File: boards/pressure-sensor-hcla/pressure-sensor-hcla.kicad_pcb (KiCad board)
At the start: 2 copper layers, 27.5 x 19 mm, 5 parts, among them J1 CONN_01X04, M3 MountingHole_3.2mm_M3, U1 HCLA-XXXX-DIP-X

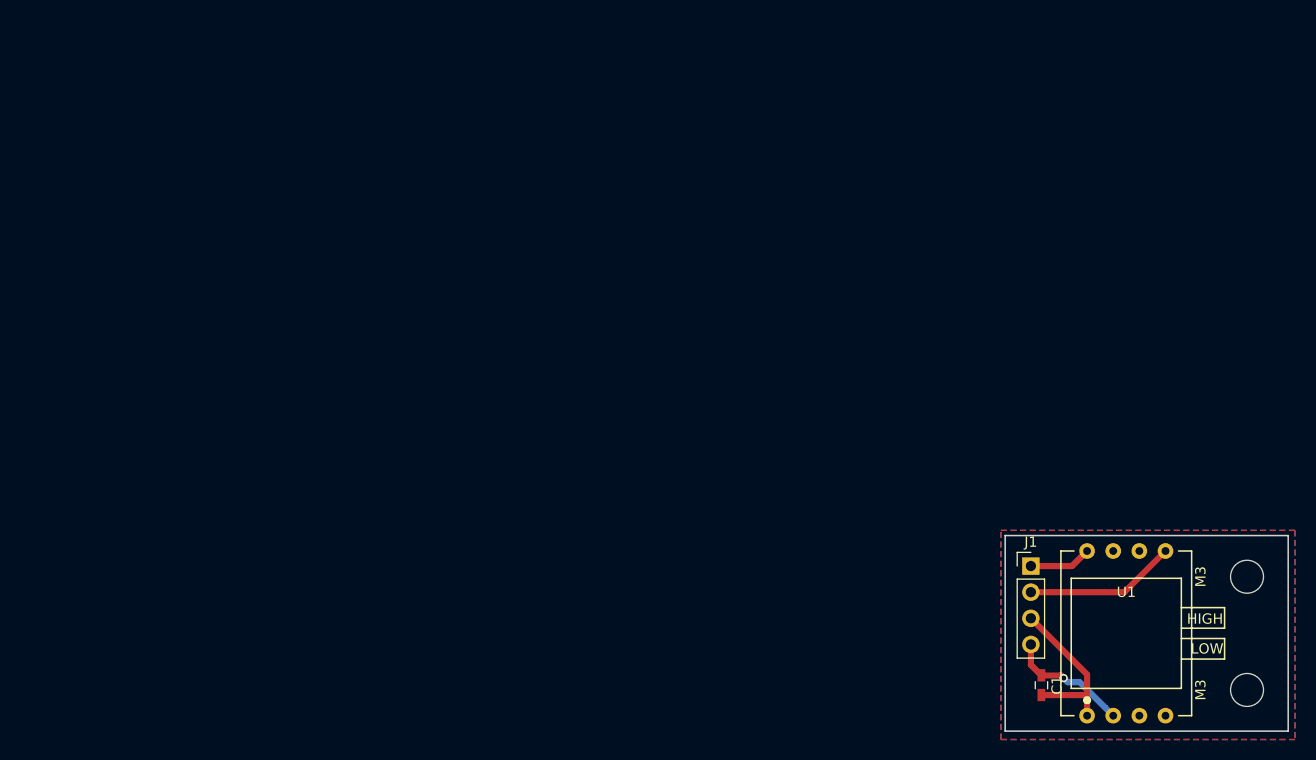
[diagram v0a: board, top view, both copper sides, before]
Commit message: [docs] export all board layouts
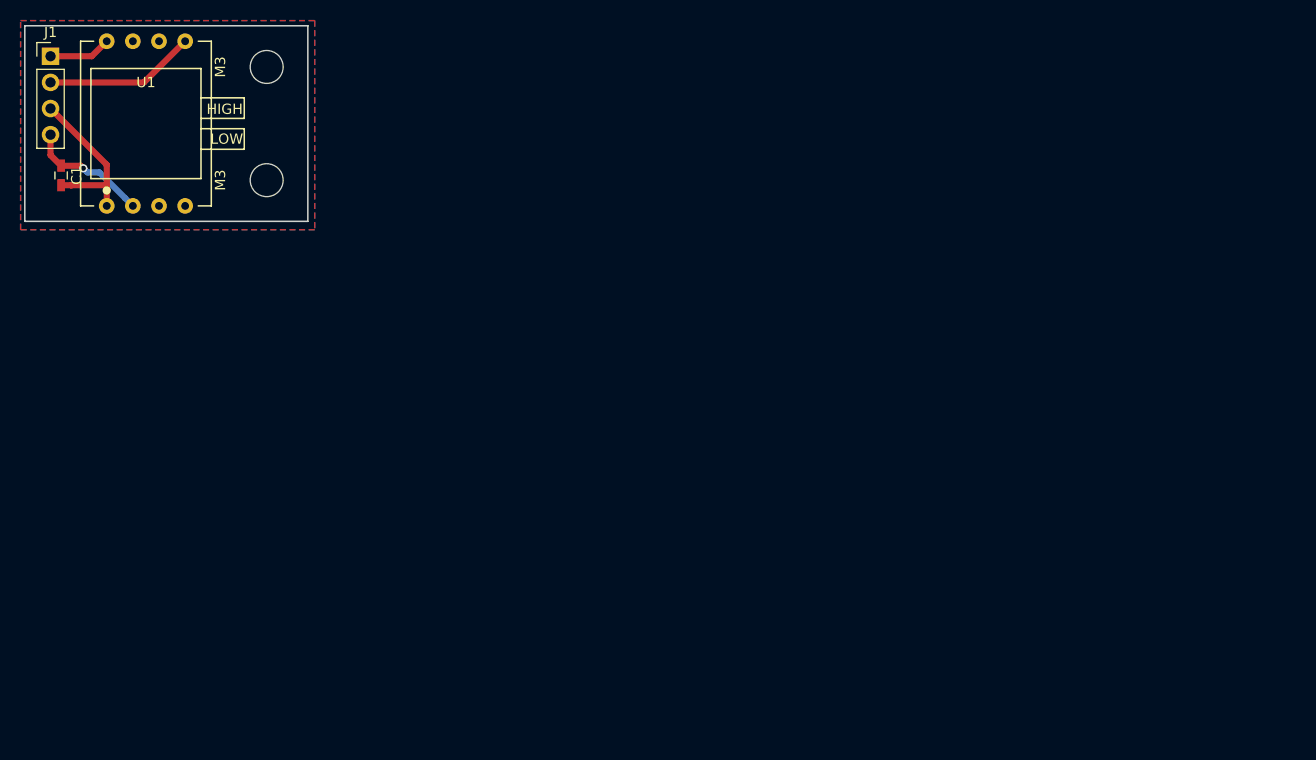
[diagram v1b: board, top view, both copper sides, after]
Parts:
- moved J1 107.4 mm to (56.2, 40.9)
- moved M3 107.4 mm to (77.2, 42.0)
- moved M3 107.4 mm to (77.2, 53.0)
- moved C1 107.4 mm to (57.3, 52.5)
- moved U1 107.4 mm to (59.2, 55.5)
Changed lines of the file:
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@@
   (general
     (links 6)
-    (no_connects 1)
+    (no_connects 0)
     (area 147.025 85.525 182.057143 109.075)
     (thickness 1.6)
@@
     (nets 5)
   )
-  (page A4)
+  (page User 140.005 119.99)
+  (title_block
+    (title "Pressure sensor board HCLA")
+    (date 2017-05-21)
+    (rev 1)
+    (company VIPER)
+  )
   (layers
     (0 F.Cu signal)
@@
   )
   (module Capacitors_SMD:C_0603_HandSoldering (layer F.Cu)
-    (at 152.527 102.042 90)
+    (at 57.277 52.512 90)
     (descr "Capacitor SMD 0603, hand soldering")
     (tags "capacitor 0603")
@@
   )
   (module Pin_Headers:Pin_Header_Straight_1x04_Pitch2.54mm (layer F.Cu)
-    (at 151.5 90.46)
+    (at 56.25 40.93)
     (descr "Through hole straight pin header, 1x04, 2.54mm pitch, single row")
     (tags "Through hole pin header THT 1x04 2.54mm single row")
@@
   )
   (module pressure-sensor-hcla:HCLA-DIP (layer F.Cu)
-    (at 154.42 105)
+    (at 59.17 55.47)
     (fp_text reference U1 (at 6.35 -12) (layer F.SilkS)
       (effects (font (size 1 1) (thickness 0.15)))
@@
   )
   (module Mounting_Holes:MountingHole_3.2mm_M3 (layer F.Cu)
-    (at 172.5 91.5)
+    (at 77.25 41.97)
     (descr "Mounting Hole 3.2mm, no annular, M3")
     (tags "mounting hole 3.2mm no annular m3")
@@
   )
   (module Mounting_Holes:MountingHole_3.2mm_M3 (layer F.Cu)
-    (at 172.5 102.5)
+    (at 77.25 52.97)
     (descr "Mounting Hole 3.2mm, no annular, M3")
     (tags "mounting hole 3.2mm no annular m3")
@@
     (pad 1 np_thru_hole circle (at 0 0) (size 3.2 3.2) (drill 3.2) (layers *.Cu *.Mask))
   )
-  (gr_text GND (at 155.5 98.5) (layer B.SilkS)
-    (effects (font (size 1.5 1.5) (thickness 0.3)) (justify mirror))
-  )
-  (gr_text "rexus-viper\npressure-\nsensor-HCLA\n©rchojetzki" (at 163.5 97 90) (layer B.SilkS)
-    (effects (font (size 1.5 1.5) (thickness 0.3)) (justify mirror))
-  )
-  (gr_text VCC (at 155.5 95.5) (layer B.SilkS)
-    (effects (font (size 1.5 1.5) (thickness 0.3)) (justify mirror))
-  )
-  (gr_text SCL (at 155.5 93) (layer B.SilkS)
-    (effects (font (size 1.5 1.5) (thickness 0.3)) (justify mirror))
-  )
-  (gr_text SDA (at 155.5 90.5) (layer B.SilkS)
-    (effects (font (size 1.5 1.5) (thickness 0.3)) (justify mirror))
-  )
-  (gr_line (start 176.5 106.5) (end 176.5 87.5) (layer Edge.Cuts) (width 0.15))
-  (gr_line (start 149 106.5) (end 176.5 106.5) (layer Edge.Cuts) (width 0.15))
-  (gr_line (start 149 87.5) (end 149 106.5) (layer Edge.Cuts) (width 0.15))
-  (gr_line (start 176.5 87.5) (end 149 87.5) (layer Edge.Cuts) (width 0.15))
-  (segment (start 156.96 101) (end 156.96 102.997) (width 0.6) (layer F.Cu) (net 1))
-  (segment (start 156.96 102.997) (end 156.96 105) (width 0.6) (layer F.Cu) (net 1))
-  (segment (start 152.527 102.992) (end 153.502 102.992) (width 0.6) (layer F.Cu) (net 1))
-  (segment (start 153.502 102.992) (end 153.507 102.997) (width 0.6) (layer F.Cu) (net 1))
-  (segment (start 153.507 102.997) (end 156.96 102.997) (width 0.6) (layer F.Cu) (net 1))
-  (segment (start 151.5 95.54) (end 156.96 101) (width 0.6) (layer F.Cu) (net 1))
-  (segment (start 154.686 101.346) (end 155.085999 101.745999) (width 0.6) (layer B.Cu) (net 2))
-  (segment (start 155.085999 101.745999) (end 156.245999 101.745999) (width 0.6) (layer B.Cu) (net 2))
-  (segment (start 156.245999 101.745999) (end 158.738001 104.238001) (width 0.6) (layer B.Cu) (net 2))
-  (segment (start 158.738001 104.238001) (end 159.5 105) (width 0.6) (layer B.Cu) (net 2))
-  (segment (start 152.527 101.092) (end 154.432 101.092) (width 0.6) (layer F.Cu) (net 2))
-  (segment (start 154.432 101.092) (end 154.686 101.346) (width 0.6) (layer F.Cu) (net 2))
-  (via (at 154.686 101.346) (size 0.8) (drill 0.5) (layers F.Cu B.Cu) (net 2))
-  (segment (start 151.5 98.08) (end 151.5 100.065) (width 0.6) (layer F.Cu) (net 2))
-  (segment (start 151.5 100.065) (end 152.527 101.092) (width 0.6) (layer F.Cu) (net 2))
-  (segment (start 151.92 98.5) (end 151.5 98.08) (width 0.6) (layer F.Cu) (net 2))
-  (segment (start 151.5 90.46) (end 155.5 90.46) (width 0.6) (layer F.Cu) (net 3))
-  (segment (start 155.5 90.46) (end 156.96 89) (width 0.6) (layer F.Cu) (net 3))
-  (segment (start 151.5 93) (end 160.58 93) (width 0.6) (layer F.Cu) (net 4))
-  (segment (start 160.58 93) (end 164.58 89) (width 0.6) (layer F.Cu) (net 4))
+  (gr_text GND (at 60.25 48.97) (layer B.SilkS)
+    (effects (font (size 1.5 1.5) (thickness 0.3)) (justify mirror))
+  )
+  (gr_text "rexus-viper\npressure-\nsensor-HCLA\n©rchojetzki" (at 68.25 47.47 90) (layer B.SilkS)
+    (effects (font (size 1.5 1.5) (thickness 0.3)) (justify mirror))
+  )
+  (gr_text VCC (at 60.25 45.97) (layer B.SilkS)
+    (effects (font (size 1.5 1.5) (thickness 0.3)) (justify mirror))
+  )
+  (gr_text SCL (at 60.25 43.47) (layer B.SilkS)
+    (effects (font (size 1.5 1.5) (thickness 0.3)) (justify mirror))
+  )
+  (gr_text SDA (at 60.25 40.97) (layer B.SilkS)
+    (effects (font (size 1.5 1.5) (thickness 0.3)) (justify mirror))
+  )
+  (gr_line (start 81.25 56.97) (end 81.25 37.97) (layer Edge.Cuts) (width 0.15))
+  (gr_line (start 53.75 56.97) (end 81.25 56.97) (layer Edge.Cuts) (width 0.15))
+  (gr_line (start 53.75 37.97) (end 53.75 56.97) (layer Edge.Cuts) (width 0.15))
+  (gr_line (start 81.25 37.97) (end 53.75 37.97) (layer Edge.Cuts) (width 0.15))
+  (segment (start 61.71 51.47) (end 61.71 53.467) (width 0.6) (layer F.Cu) (net 1))
+  (segment (start 61.71 53.467) (end 61.71 55.47) (width 0.6) (layer F.Cu) (net 1))
+  (segment (start 57.277 53.462) (end 58.252 53.462) (width 0.6) (layer F.Cu) (net 1))
+  (segment (start 58.252 53.462) (end 58.257 53.467) (width 0.6) (layer F.Cu) (net 1))
+  (segment (start 58.257 53.467) (end 61.71 53.467) (width 0.6) (layer F.Cu) (net 1))
+  (segment (start 56.25 46.01) (end 61.71 51.47) (width 0.6) (layer F.Cu) (net 1))
+  (segment (start 59.436 51.816) (end 59.835999 52.215999) (width 0.6) (layer B.Cu) (net 2))
+  (segment (start 59.835999 52.215999) (end 60.995999 52.215999) (width 0.6) (layer B.Cu) (net 2))
+  (segment (start 60.995999 52.215999) (end 63.488001 54.708001) (width 0.6) (layer B.Cu) (net 2))
+  (segment (start 63.488001 54.708001) (end 64.25 55.47) (width 0.6) (layer B.Cu) (net 2))
+  (segment (start 57.277 51.562) (end 59.182 51.562) (width 0.6) (layer F.Cu) (net 2))
+  (segment (start 59.182 51.562) (end 59.436 51.816) (width 0.6) (layer F.Cu) (net 2))
+  (via (at 59.436 51.816) (size 0.8) (drill 0.5) (layers F.Cu B.Cu) (net 2))
+  (segment (start 56.25 48.55) (end 56.25 50.535) (width 0.6) (layer F.Cu) (net 2))
+  (segment (start 56.25 50.535) (end 57.277 51.562) (width 0.6) (layer F.Cu) (net 2))
+  (segment (start 56.67 48.97) (end 56.25 48.55) (width 0.6) (layer F.Cu) (net 2))
+  (segment (start 56.25 40.93) (end 60.25 40.93) (width 0.6) (layer F.Cu) (net 3))
+  (segment (start 60.25 40.93) (end 61.71 39.47) (width 0.6) (layer F.Cu) (net 3))
+  (segment (start 56.25 43.47) (end 65.33 43.47) (width 0.6) (layer F.Cu) (net 4))
+  (segment (start 65.33 43.47) (end 69.33 39.47) (width 0.6) (layer F.Cu) (net 4))
   (zone (net 0) (net_name "") (layer F.Cu) (hatch edge 0.508)
     (connect_pads (clearance 0.508))
@@
     (polygon
       (pts
-        (xy 171 99) (xy 174 99) (xy 176 101) (xy 176 102.5) (xy 176 104)
-        (xy 174 106) (xy 171 106) (xy 169 104) (xy 169 100.5)
+        (xy 75.75 49.47) (xy 78.75 49.47) (xy 80.75 51.47) (xy 80.75 52.97) (xy 80.75 54.47)
+        (xy 78.75 56.47) (xy 75.75 56.47) (xy 73.75 54.47) (xy 73.75 50.97)
       )
     )
@@
     (polygon
       (pts
-        (xy 171 99) (xy 174 99) (xy 176 101) (xy 176 104) (xy 174 106)
-        (xy 171 106) (xy 169 104) (xy 169 100.5)
+        (xy 75.75 49.47) (xy 78.75 49.47) (xy 80.75 51.47) (xy 80.75 54.47) (xy 78.75 56.47)
+        (xy 75.75 56.47) (xy 73.75 54.47) (xy 73.75 50.97)
       )
     )
@@
     (polygon
       (pts
-        (xy 171 88) (xy 174 88) (xy 176 90) (xy 176 93) (xy 174 95)
-        (xy 171 95) (xy 169 93) (xy 169 90)
+        (xy 75.75 38.47) (xy 78.75 38.47) (xy 80.75 40.47) (xy 80.75 43.47) (xy 78.75 45.47)
+        (xy 75.75 45.47) (xy 73.75 43.47) (xy 73.75 40.47)
       )
     )
@@
     (polygon
       (pts
-        (xy 171 88) (xy 174 88) (xy 176 90) (xy 176 93) (xy 174 95)
-        (xy 171 95) (xy 169 93) (xy 169 90)
+        (xy 75.75 38.47) (xy 78.75 38.47) (xy 80.75 40.47) (xy 80.75 43.47) (xy 78.75 45.47)
+        (xy 75.75 45.47) (xy 73.75 43.47) (xy 73.75 40.47)
       )
     )
@@
     (polygon
       (pts
-        (xy 148.59 86.995) (xy 177.165 86.995) (xy 177.165 107.315) (xy 148.59 107.315)
+        (xy 53.34 37.465) (xy 81.915 37.465) (xy 81.915 57.785) (xy 53.34 57.785)
       )
     )
@@
     (polygon
       (pts
-        (xy 148.59 86.995) (xy 177.165 86.995) (xy 177.165 107.315) (xy 148.59 107.315)
-      )
-    )
+        (xy 53.34 37.465) (xy 81.915 37.465) (xy 81.915 57.785) (xy 53.34 57.785)
+      )
+    )
